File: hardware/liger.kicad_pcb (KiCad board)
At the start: 2 copper layers, 33.1 x 92.2 mm, 55 parts, among them J1 Conn_02x08_Odd_Even, Q1 Q_NPN_BEC, Q4 PMOS-DMG3413L, U1 ESP-WROOM-32, U12 soft-button-4x, U2 IR-RX-TSOP34438, U3 SPH0645LM4H-B, U4 MCP73831T, U5 MAX98357AETE+T, U6 SI7020-A20, U7 PYQ2898, U8 TSL45315CL, U9 AP2112

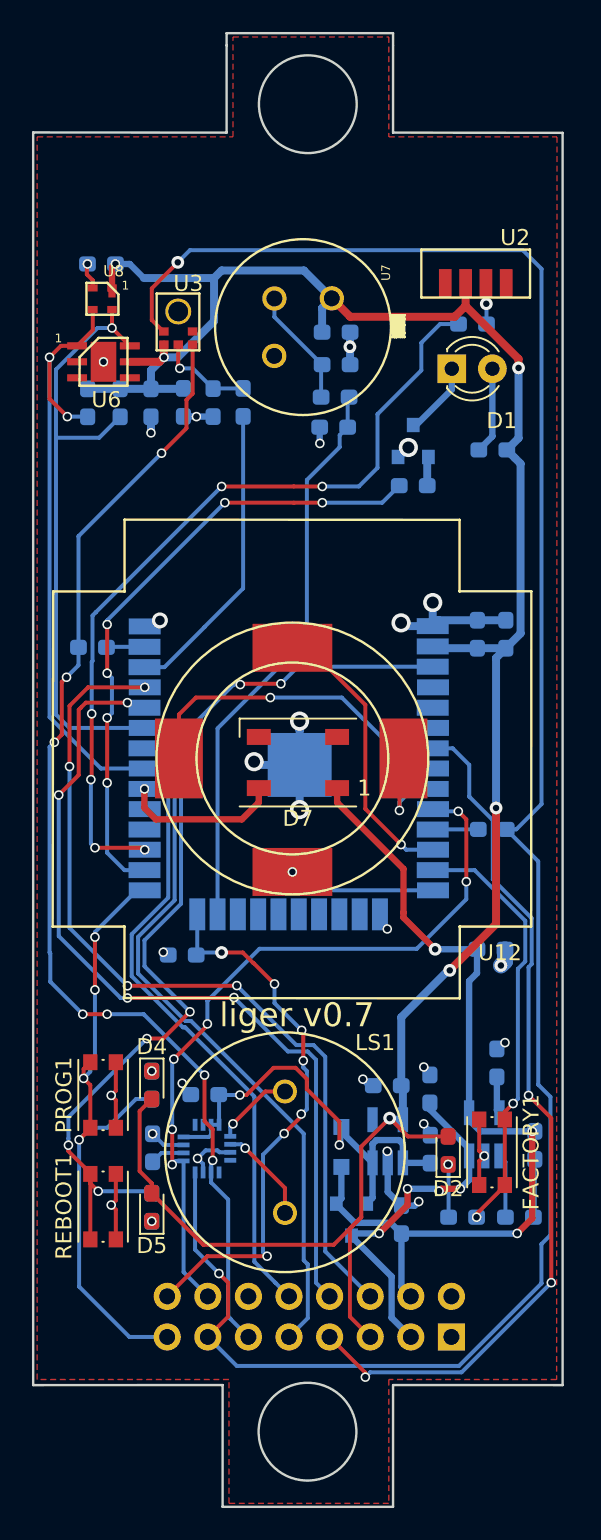
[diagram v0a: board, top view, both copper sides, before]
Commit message: update button
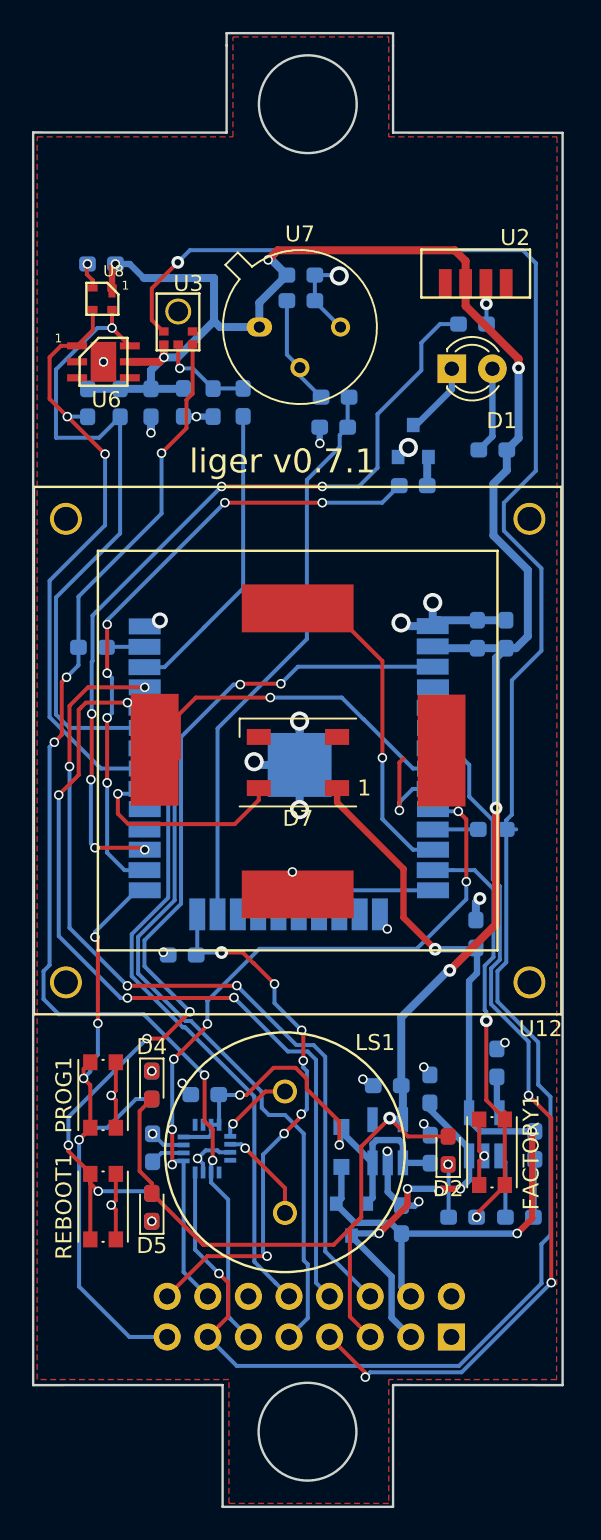
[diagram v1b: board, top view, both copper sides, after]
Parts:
- added LOGO: , open-automation:pyfi_symbol, B.Cu at (157.2, 50.9)
- U7: footprint open-automation:PYQ2898 -> Package_TO_SOT_THT:TO-5-3
- moved C4 4.57 mm to (147.2, 59.8)
- moved C3 4.20 mm to (147.2, 58.1)
- moved U7 2.73 mm to (144.7, 61.4), turned to 0 degrees
- moved C12 1.34 mm to (158.2, 99.4), turned to 270 degrees
- moved U12 0.59 mm to (147.1, 87.9)
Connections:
- U7 pad 2: GND -> Net-(C4-Pad1)
- U7 pad 3: Net-(C4-Pad1) -> GND
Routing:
- net /3V3: track 150.8 -> 155.3 mm, vias 6 -> 7
- net GND: track 56.6 -> 60.3 mm
- net /SCL: track 85.4 -> 89.0 mm
- net /BUTTON_LED: track 9.97 -> 13.5 mm
- net /T_UP: track 17.8 -> 20.5 mm
- net /I2S_BCLK: track 131.2 -> 133.6 mm
- net /SDA: track 79.4 -> 78.1 mm
- net /I2S_WS: track 73.3 -> 74.5 mm, vias 7 -> 5
- net Net-(C4-Pad1): track 7.43 -> 6.92 mm
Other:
- board text added: "liger v0.7.1"
- board text removed: "liger v0.7"
